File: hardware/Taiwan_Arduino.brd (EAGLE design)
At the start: 97.2 x 35.7 mm, 44 parts, among them J1 AVR_SPI_PRG_62X3_LOCK, T1 2SC, T2 2N, U1 ATMEGA328P_PDIP, Y2 16mhz

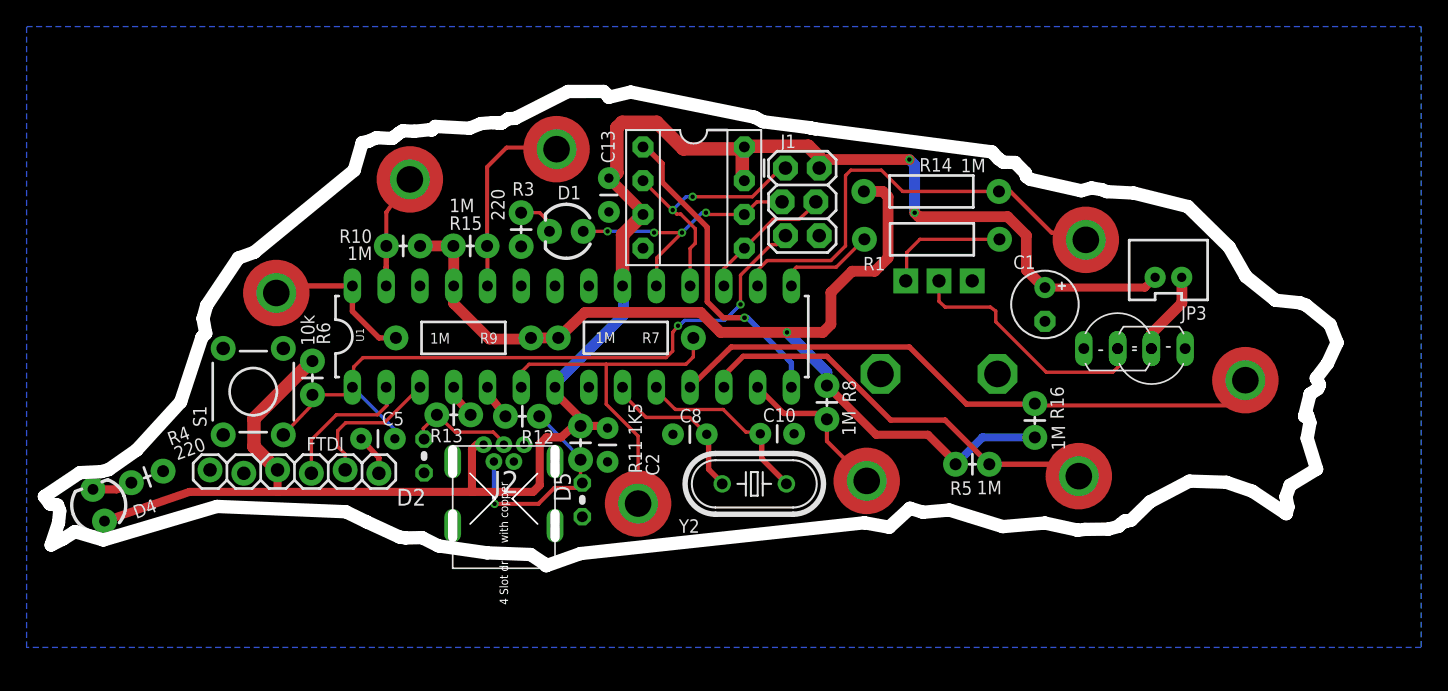
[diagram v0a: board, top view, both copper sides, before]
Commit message: Ver 1.0
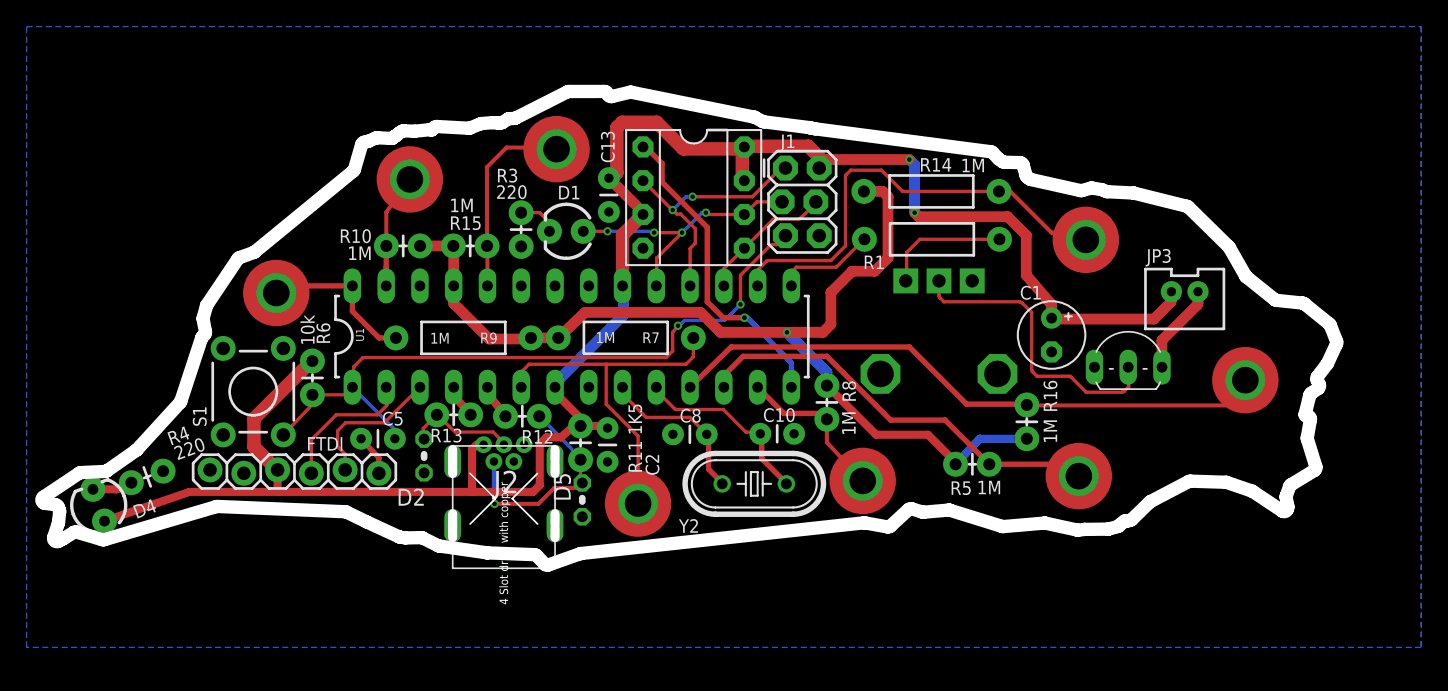
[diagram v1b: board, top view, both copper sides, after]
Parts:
- removed T1: 2SC, transistor:TO92-ECB
- moved JP3 2.50 mm to (87.4, 23.5), turned to 180 degrees
- moved C1 2.35 mm to (77.4, 20.8)
- moved T2 1.61 mm to (83.2, 19.7)
- moved R16 0.61 mm to (75.5, 13.0)
- moved TP6 0.30 mm to (63.2, 9.83)
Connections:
- removed net N$18: JP3.2, T1.C, T2.C
- new net N$12: JP3.1, T2.C
- net +5V: now also JP3.2; no longer JP3.1
- net GND: no longer T1.E
- net N$22: no longer T1.B
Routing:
- net N$12: track 0.00 -> 6.79 mm
- net N$18: track 6.31 -> 0.00 mm
- net +5V: track 140.1 -> 144.2 mm
- net N$22: track 19.2 -> 22.6 mm
- net N$17: track 47.1 -> 48.2 mm
- net N$11: track 76.6 -> 76.0 mm
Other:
- board size 97.2 x 35.7 mm -> 97.4 x 35.6 mm

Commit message: ver 1.0
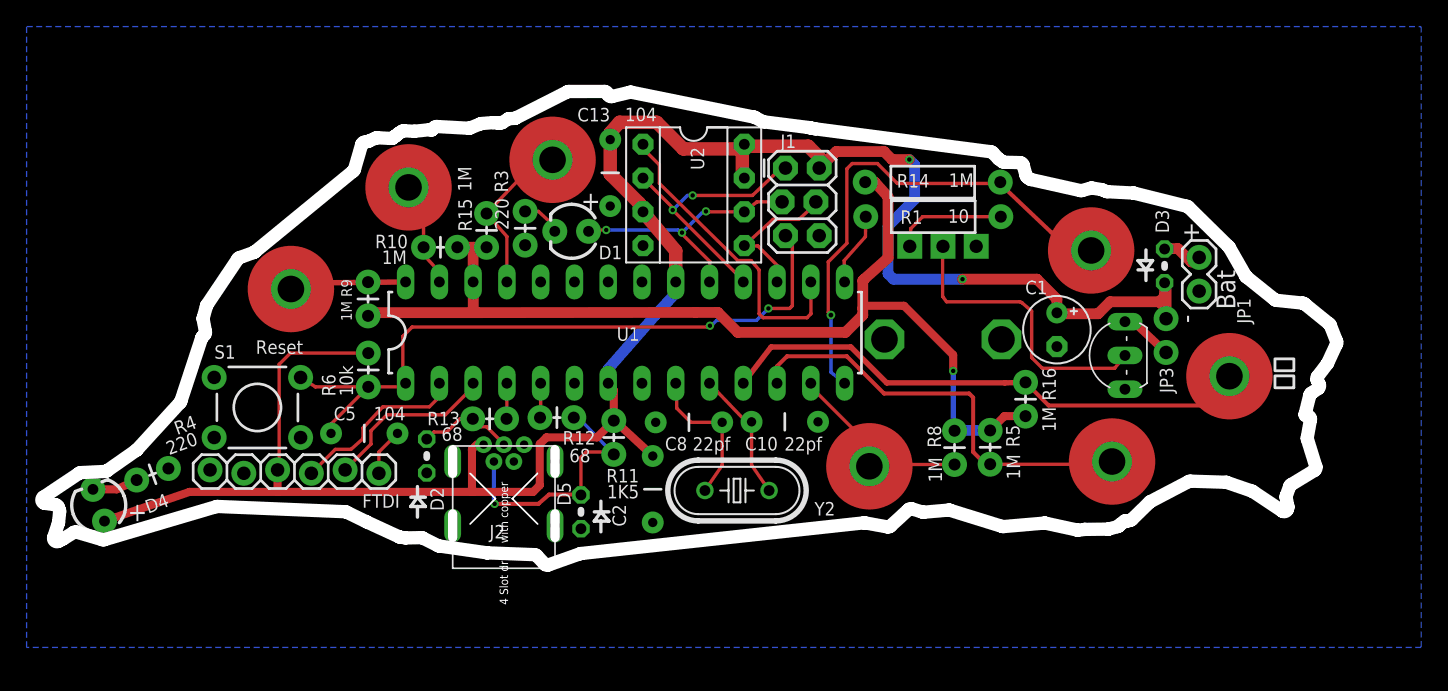
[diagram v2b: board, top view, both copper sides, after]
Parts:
- removed R7: 1M, SparkFun-Resistors:AXIAL-0.4
- removed TP5: TEST-POINT, SparkFun-Passives:PADBIG
- removed U$1: SPI_FLASH-X25XX, SparkFun-DigitalIC:DIL08
- added D3: 3.3V, _JJG-parts:0204V
- added JP1: Battery, SparkFun-Connectors:1X02
- added U2: SPI_FLASH, SparkFun-DigitalIC:DIL08
- C10, C13, C5, C8: device SparkFun-Capacitors:CAP-PTH-SMALL -> SparkFun-Capacitors:CAP-PTH-5MM
- C2: value 0.1uf -> 104; device SparkFun-Capacitors:CAP-PTH-SMALL -> SparkFun-Capacitors:CAP-PTH-5MM
- JP3: value M02JST-PTH-VERT -> M021X02_NO_SILK; device SparkFun-Connectors:JST-2-PTH-VERT -> SparkFun-Connectors:1X02_NO_SILK
- R1: value (none) -> 10
- R9: device SparkFun-Resistors:AXIAL-0.4 -> SparkFun-Resistors:AXIAL-0.1
- T2: value 2N -> 2N2222
- moved R8 10.2 mm to (70.1, 13.6)
- moved R9 7.37 mm to (26.0, 22.2), turned to 90 degrees
- moved C2 5.72 mm to (47.4, 9.20)
- moved JP3 4.26 mm to (86.0, 19.5), turned to 90 degrees
- moved R6 4.24 mm to (26.0, 16.9)
- moved U1 4.01 mm to (45.3, 21.0)
- moved R5 3.64 mm to (72.8, 13.6), turned to 270 degrees
- moved R10 2.80 mm to (32.7, 27.4)
- moved TP3 2.73 mm to (81.9, 11.3)
- moved R13 2.72 mm to (36.4, 14.5)
- moved RV1 2.62 mm to (69.2, 20.5)
- moved R12 2.60 mm to (38.9, 14.6)
- moved R11 2.53 mm to (44.5, 11.8)
- moved R15 2.50 mm to (34.9, 27.4), turned to 90 degrees
- moved C5 2.33 mm to (25.7, 13.4), turned to 0 degrees
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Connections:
- removed net N$27: R7.P$2, TP5.P$1, U1.6
- new net N$18: D3.1, JP1.2
- net +5V: now also D3.2, U2.3, U2.7, U2.8; no longer U$1.3, U$1.7, U$1.8
- net GND: now also JP1.1, U2.4; no longer U$1.4
- net N$10: now also U2.2; no longer U$1.2
- net N$11: now also U1.26; no longer R7.P$1, U1.25
- net N$23: now also U2.5; no longer U$1.5
- net N$28: now also U1.16, U2.1; no longer U$1.1, U1.14
- net N$3: now also U1.14; no longer U1.16
- net N$5: now also U1.25; no longer U1.24
- net N$6: now also U2.6; no longer U$1.6
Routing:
- net N$27: track 27.5 -> 0.00 mm
- net +5V: track 144.2 -> 159.4 mm
- net 1: track 11.9 -> 17.9 mm
- net N$17: track 48.2 -> 42.8 mm
- net N$3: track 35.4 -> 39.9 mm, vias 0 -> 1
- net N$13: track 14.0 -> 10.0 mm
- net N$18: track 0.00 -> 3.71 mm
- net N$11: track 76.0 -> 79.2 mm
- net N$9: track 10.7 -> 13.5 mm
- net N$12: track 6.79 -> 4.01 mm
- net N$15: track 17.1 -> 19.6 mm
- net N$5: track 14.9 -> 12.4 mm
- net N$14: track 10.7 -> 13.1 mm
- net N$2: track 7.57 -> 5.53 mm
- net N$29: track 31.7 -> 33.6 mm
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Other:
- board text added: "+"
- board text added: "-"
- board text added: "104"
- board text added: "22pf"
- board text added: "Bat"
- board text added: "Reset"
- board text added: "台灣"
